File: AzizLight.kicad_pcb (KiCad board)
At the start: 2 copper layers, 70.1 x 29.2 mm, 58 parts, among them P1 +9V, Q1 BS170, Q2 BS170, Q3 BS170, Q4 BS170, SW1 Reset, SW2 Invert, U1 MCP602, U2 LM393, U3 MCP601, U4 MC7805

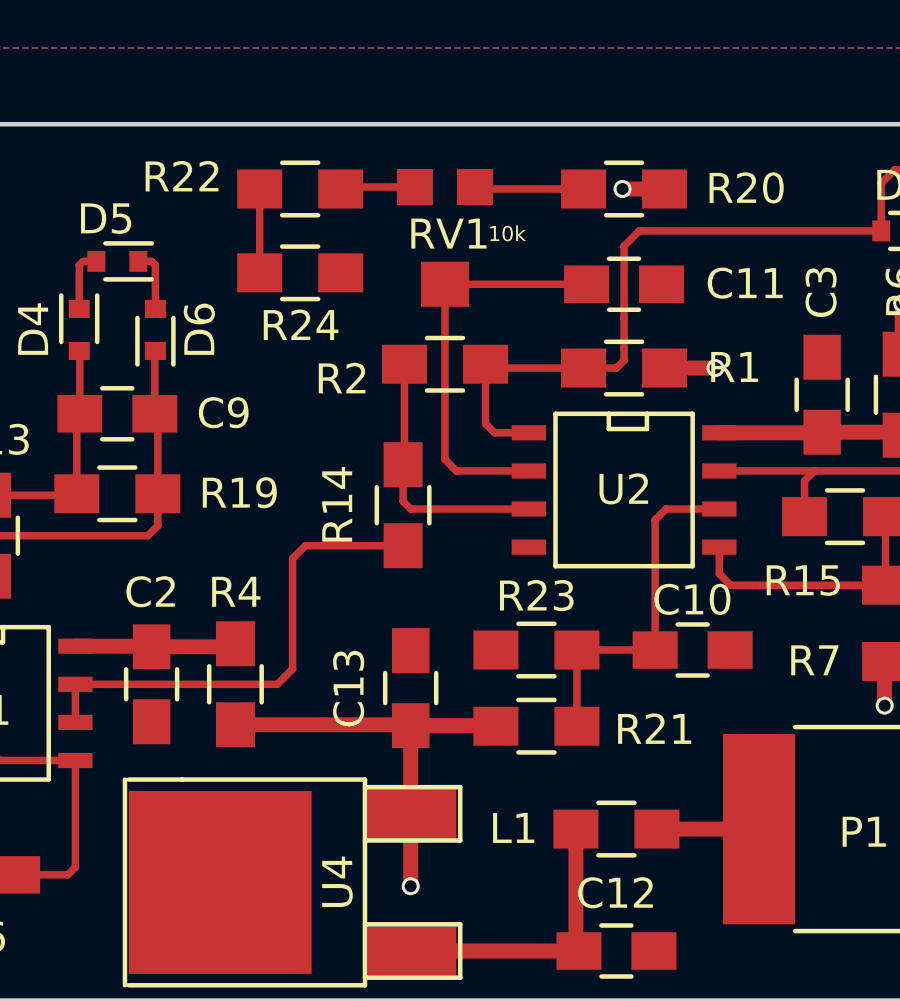
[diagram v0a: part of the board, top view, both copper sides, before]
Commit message: Updated README
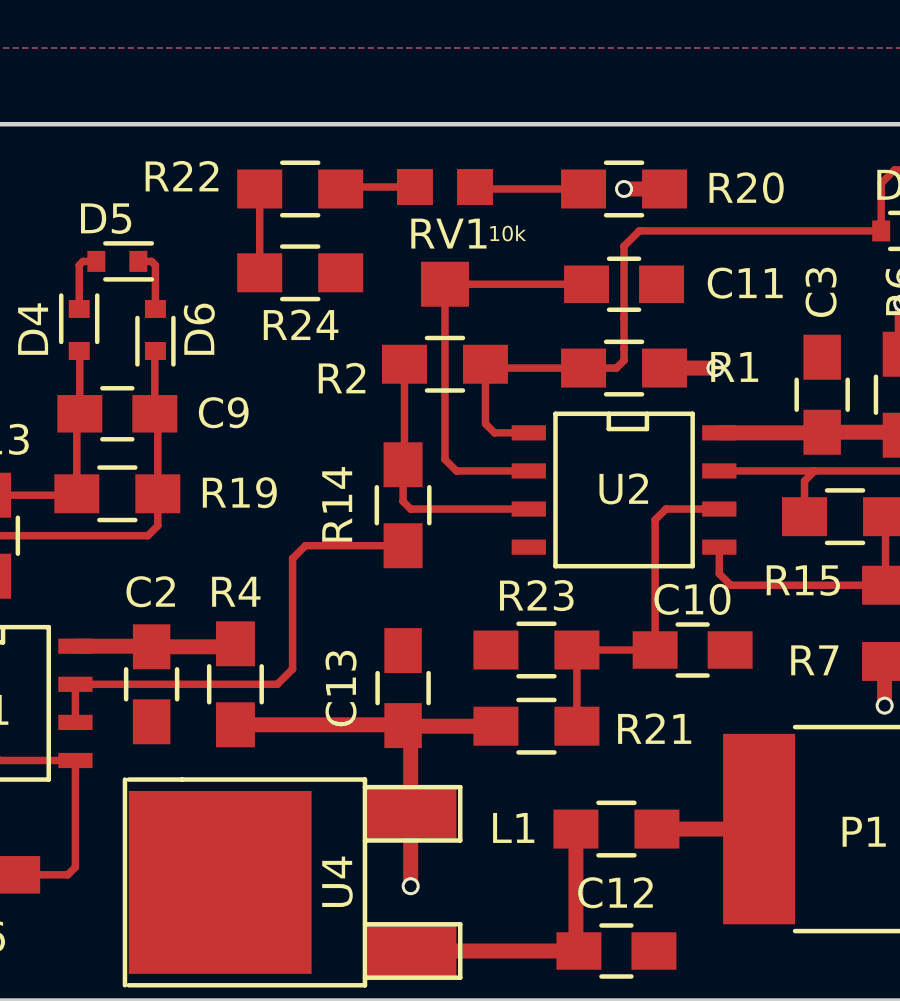
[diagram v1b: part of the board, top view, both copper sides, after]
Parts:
- moved C13 0.25 mm to (141.7, 95.4)
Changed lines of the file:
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@@
     (thickness 1.6)
     (drawings 20)
-    (tracks 215)
+    (tracks 218)
     (zones 0)
     (modules 58)
@@
   )
   (module Capacitors_SMD:C_0805_HandSoldering (layer F.Cu)
-    (at 141.986 95.377 90)
+    (at 141.732 95.377 90)
     (descr "Capacitor SMD 0805, hand soldering")
     (tags "capacitor 0805")
@@
   (segment (start 147.494 100.076) (end 147.494 104.04) (width 0.5) (layer F.Cu) (net 14))
   (segment (start 147.494 104.04) (end 147.594 104.14) (width 0.5) (layer F.Cu) (net 14))
+  (segment (start 150.448 78.74) (end 149.098 78.74) (width 0.5) (layer F.Cu) (net 15))
+  (via (at 149.098 78.74) (size 0.6) (drill 0.4) (layers F.Cu B.Cu) (net 15))
+  (segment (start 144.827 96.647) (end 141.752 96.647) (width 0.5) (layer F.Cu) (net 15))
+  (segment (start 141.752 96.647) (end 141.732 96.627) (width 0.5) (layer F.Cu) (net 15))
+  (segment (start 136.144 96.6) (end 141.705 96.6) (width 0.5) (layer F.Cu) (net 15))
+  (segment (start 141.705 96.6) (end 141.732 96.627) (width 0.5) (layer F.Cu) (net 15))
+  (segment (start 141.986 99.568) (end 141.986 96.881) (width 0.5) (layer F.Cu) (net 15))
+  (segment (start 141.986 96.881) (end 141.732 96.627) (width 0.5) (layer F.Cu) (net 15))
   (segment (start 157.781 94.488) (end 157.781 95.9574) (width 0.5) (layer F.Cu) (net 15))
   (via (at 157.7848 95.9612) (size 0.6) (drill 0.4) (layers F.Cu B.Cu) (net 15))
@@
   (segment (start 158.369 84.248) (end 158.369 82.55) (width 0.5) (layer F.Cu) (net 15))
   (via (at 158.369 82.55) (size 0.6) (drill 0.4) (layers F.Cu B.Cu) (net 15))
-  (segment (start 141.986 96.627) (end 144.807 96.627) (width 0.5) (layer F.Cu) (net 15))
   (segment (start 144.807 96.627) (end 144.827 96.647) (width 0.5) (layer F.Cu) (net 15))
-  (segment (start 141.986 96.627) (end 141.986 99.568) (width 0.5) (layer F.Cu) (net 15))
-  (segment (start 136.144 96.6) (end 141.959 96.6) (width 0.5) (layer F.Cu) (net 15))
   (segment (start 141.959 96.6) (end 141.986 96.627) (width 0.5) (layer F.Cu) (net 15))
   (segment (start 141.986 99.568) (end 141.986 101.981) (width 0.5) (layer F.Cu) (net 15))
@@
   (via (at 172.6438 93.7006) (size 0.6) (drill 0.4) (layers F.Cu B.Cu) (net 15))
   (segment (start 172.64 93.6968) (end 172.6438 93.7006) (width 0.5) (layer F.Cu) (net 15))
-  (segment (start 150.448 78.74) (end 149.0472 78.74) (width 0.5) (layer F.Cu) (net 15))
-  (via (at 149.0472 78.74) (size 0.6) (drill 0.4) (layers F.Cu B.Cu) (net 15))
   (segment (start 117.903 98.552) (end 117.903 96.9302) (width 0.5) (layer F.Cu) (net 15))
   (via (at 117.9068 96.9264) (size 0.6) (drill 0.4) (layers F.Cu B.Cu) (net 15))
